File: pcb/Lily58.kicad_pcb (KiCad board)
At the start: 2 copper layers, 142.5 x 106.3 mm, 132 parts, among them J2 4PIN, J3 Conn_01x06_Female, J4 Conn_01x06_Female, P1 i2c_pin, P2 i2c_pin, SW1 SW_PUSH, SW10 SW_PUSH, SW11 SW_PUSH, SW12 SW_PUSH, SW13 SW_PUSH, SW14 SW_PUSH, SW15 SW_PUSH, SW16 SW_PUSH, SW17 SW_PUSH, SW18 SW_PUSH, SW19 SW_PUSH, SW2 SW_PUSH, SW20 SW_PUSH, SW21 SW_PUSH, SW22 SW_PUSH, SW23 SW_PUSH, SW24 SW_PUSH, SW25 SW_PUSH, SW26 SW_PUSH, SW27 SW_PUSH, SW28 SW_PUSH, SW29 SW_PUSH, SW3 SW_PUSH, SW4 SW_PUSH, SW5 SW_PUSH, SW6 SW_PUSH, SW7 SW_PUSH, SW8 SW_PUSH, SW9 SW_PUSH, U1 ProMicro

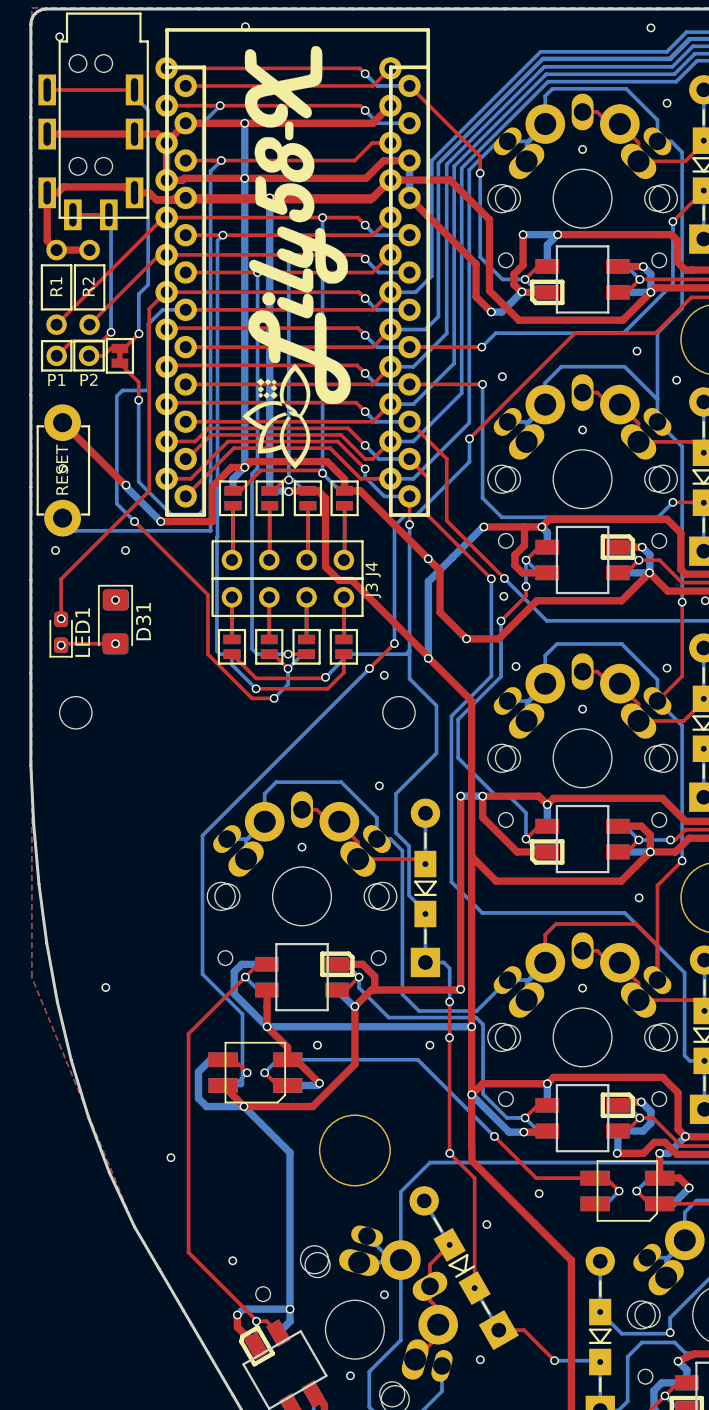
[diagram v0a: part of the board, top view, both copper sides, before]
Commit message: change 3.5mm jack assign
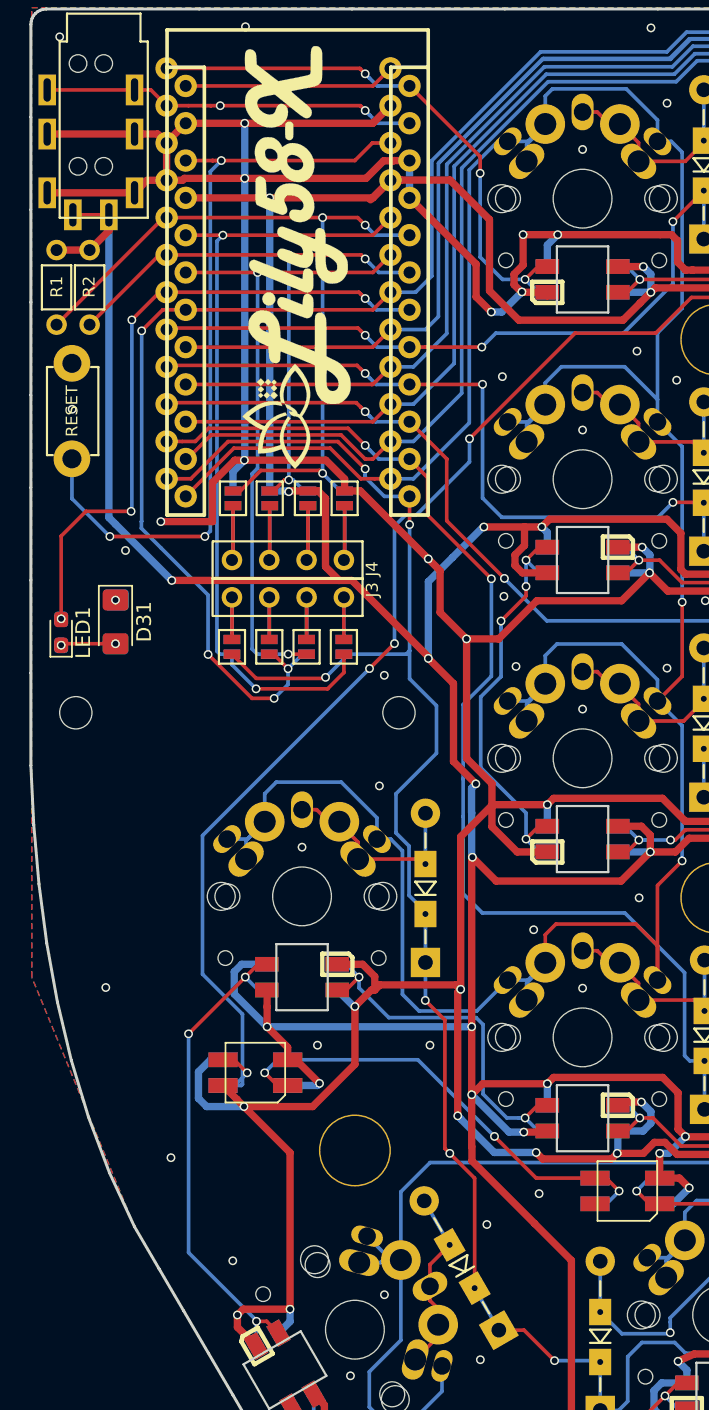
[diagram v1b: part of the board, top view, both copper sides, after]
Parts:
- removed P1, P2: i2c_pin, Lily58-footprint:1pin_conn
- removed W1: jumper, Lily58-footprint:jumper_data
- moved RSW1 4.09 mm to (85.7, 64.5)
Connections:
- J2 pad 1: VCC -> GND
- J2 pad 3: Net-(J2-Pad3) -> DATA
- J2 pad 4: Net-(J2-Pad4) -> VCC
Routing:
- net DATA: track 59.1 -> 25.6 mm, vias 3 -> 2
- net GND: track 1051.5 -> 1081.3 mm, vias 165 -> 164
- net Net-(J2-Pad3): track 26.7 -> 0.00 mm, vias 1 -> 0
- net VCC: track 1082.9 -> 1098.0 mm, vias 66 -> 69
- net Net-(J2-Pad4): track 14.8 -> 0.00 mm, vias 1 -> 0
- net RESET: track 50.5 -> 53.4 mm, vias 1 -> 3
- net col0: track 312.5 -> 310.1 mm, vias 5 -> 6
- net Net-(LED1-Pad2): track 42.2 -> 44.3 mm, vias 2 -> 4
- net Net-(L13-Pad3): track 28.9 -> 27.1 mm
- net row4: track 158.7 -> 158.0 mm, vias 7 -> 6
- net row3: track 181.1 -> 180.4 mm
- net Net-(L25-Pad1): vias 2 -> 3

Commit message: Revert "change 3.5mm jack assign"
This reverts commit aa684eaece7f45b972ff72976500a763c7363c79.
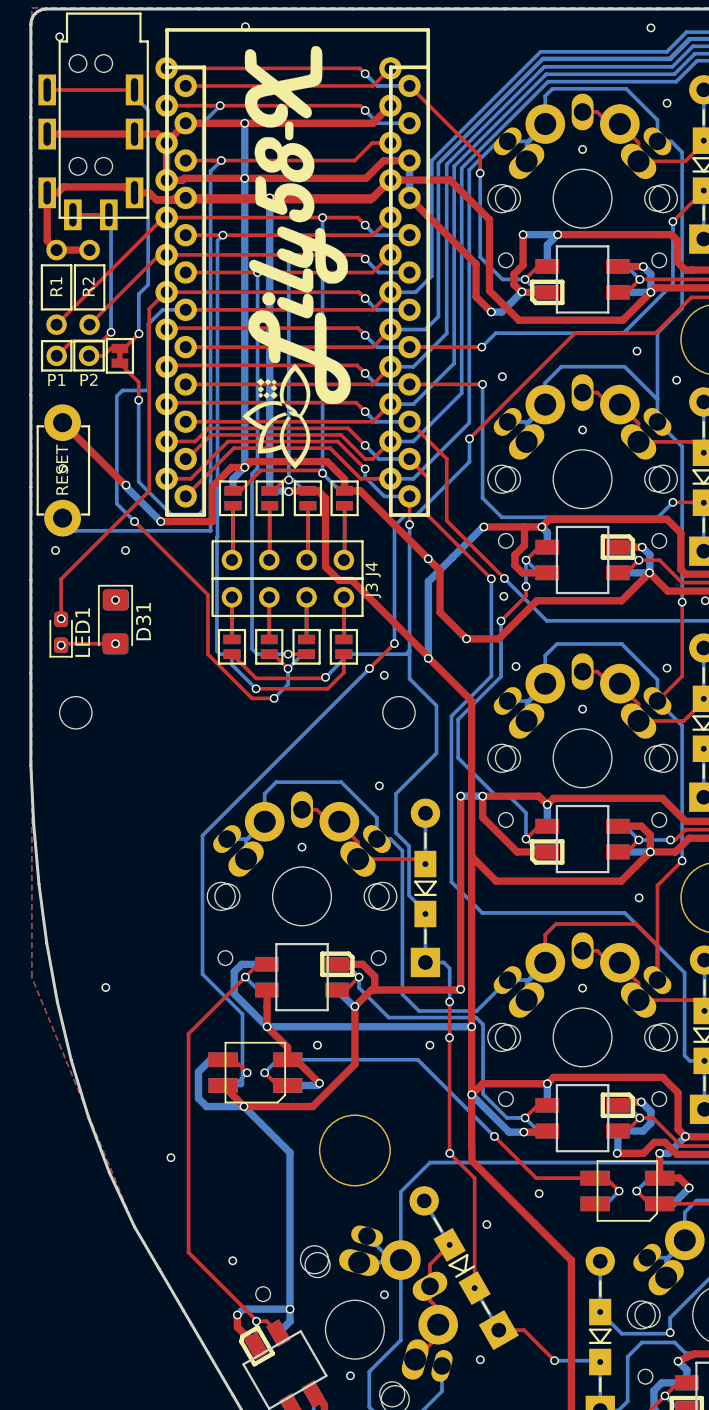
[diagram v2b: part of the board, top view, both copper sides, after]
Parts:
- added P1: i2c_pin, Lily58-footprint:1pin_conn, F.Cu at (84.7, 60.7)
- added P2: i2c_pin, Lily58-footprint:1pin_conn, F.Cu at (86.9, 60.7)
- added W1: jumper, Lily58-footprint:jumper_data, F.Cu at (89.0, 60.7)
- moved RSW1 4.09 mm to (85.1, 68.5)
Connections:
- J2 pad 1: GND -> VCC
- J2 pad 3: DATA -> Net-(J2-Pad3)
- J2 pad 4: VCC -> Net-(J2-Pad4)
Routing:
- net DATA: track 25.6 -> 59.1 mm, vias 2 -> 3
- net GND: track 1081.3 -> 1051.5 mm, vias 164 -> 165
- net Net-(J2-Pad3): track 0.00 -> 26.7 mm, vias 0 -> 1
- net VCC: track 1098.0 -> 1082.9 mm, vias 69 -> 66
- net Net-(J2-Pad4): track 0.00 -> 14.8 mm, vias 0 -> 1
- net RESET: track 53.4 -> 50.5 mm, vias 3 -> 1
- net col0: track 310.1 -> 312.5 mm, vias 6 -> 5
- net Net-(LED1-Pad2): track 44.3 -> 42.2 mm, vias 4 -> 2
- net Net-(L13-Pad3): track 27.1 -> 28.9 mm
- net row4: track 158.0 -> 158.7 mm, vias 6 -> 7
- net row3: track 180.4 -> 181.1 mm
- net Net-(L25-Pad1): vias 3 -> 2
